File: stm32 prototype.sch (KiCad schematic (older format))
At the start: 117 parts, among them J1 USB_B_Mini, J3 Conn_01x02, Q1 Q_NMOS_GSD, Q2 Q_NMOS_GSD, Q3 Q_NMOS_GSD, Q4 Q_NMOS_GSD, Q5 Q_NMOS_GSD, Q6 Q_NMOS_GSD, Q7 Q_NMOS_GSD, Q8 Q_NMOS_GSD, Q9 Q_NMOS_GSD, U1 FT232RL, U2 W25Q128JV-DTR, U3 STM32F407VGTx, U4 LD1117S33TR, U5 ESP32, U6 IS25LP016D-JNLE-TR, Y1 Crystal_GND24, Y2 Crystal_GND23, Y3 Crystal_GND23

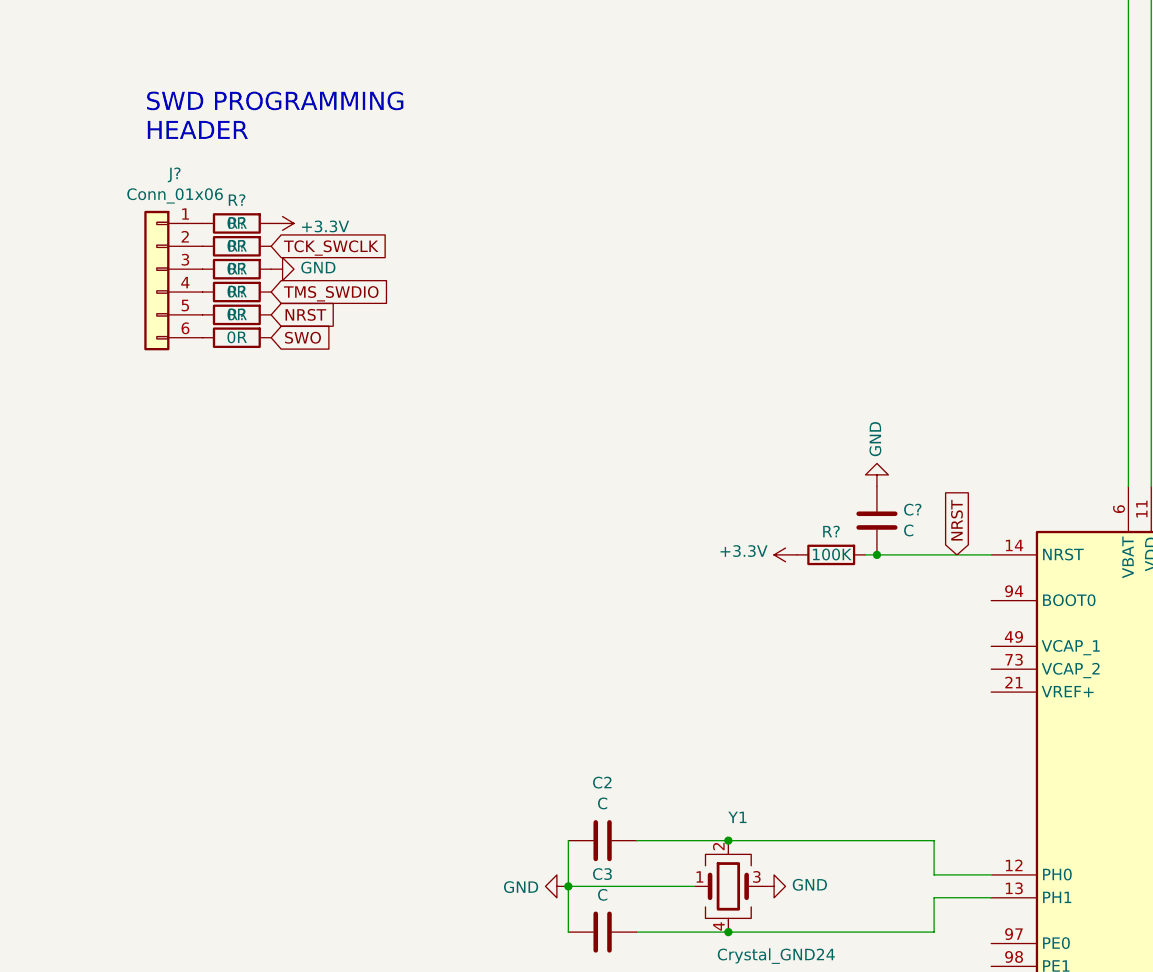
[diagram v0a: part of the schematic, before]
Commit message: worked on some layout
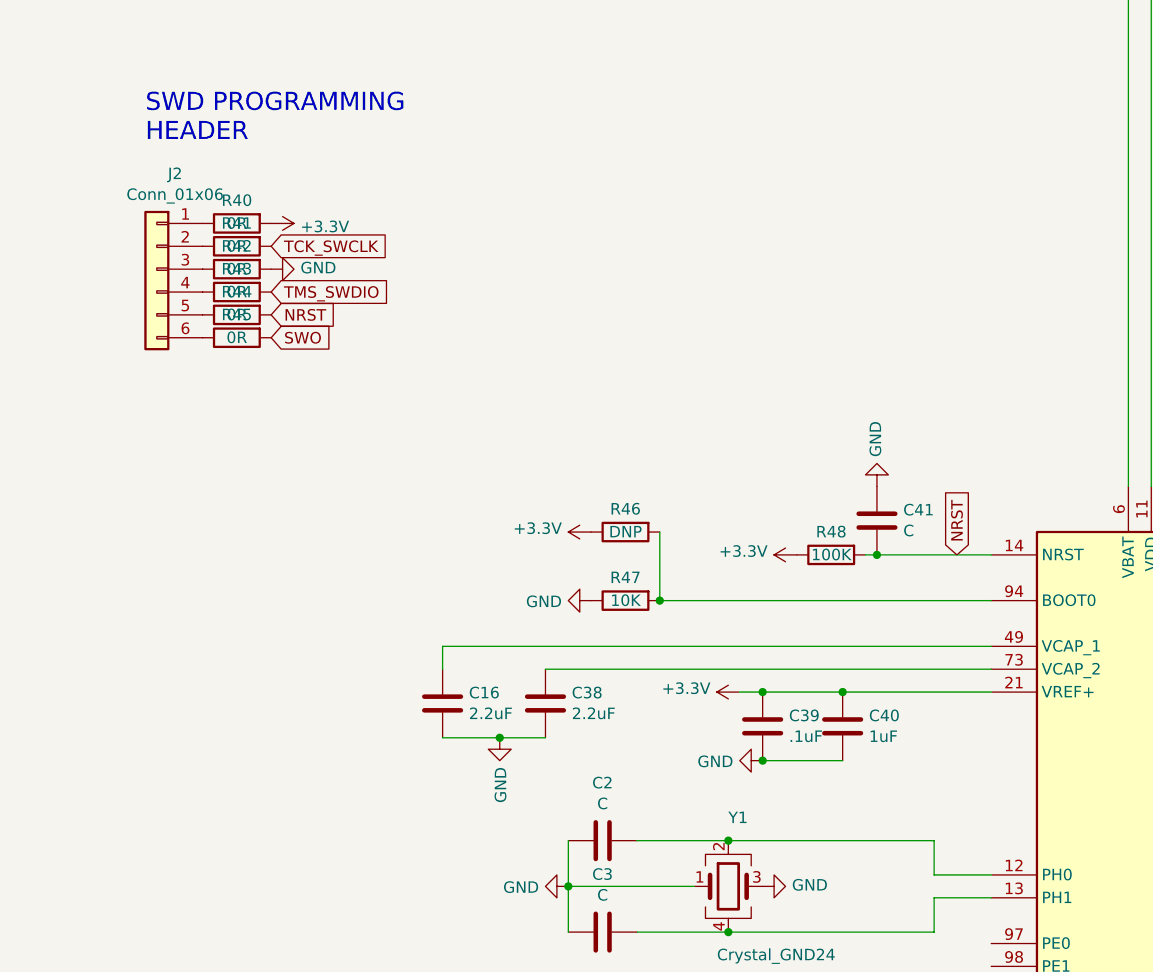
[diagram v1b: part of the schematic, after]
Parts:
- added C16, C38: 2.2uF, Capacitors_SMD:C_0603, symbol Device:C
- added C39: .1uF, Capacitors_SMD:C_0603, symbol Device:C
- added C40: 1uF, Capacitors_SMD:C_0603, symbol Device:C
- added R46: DNP, Resistors_SMD:R_0603, symbol Device:R
- added R47: 10K, Resistors_SMD:R_0603, symbol Device:R
- C1, C10, C11, C12, C13, C14, C15, C17, C18, C19, C2, C20, C21, C22, C23, C24, C25, C26, C27, C28, C29, C3, C31, C36, C37, C4, C5, C6, C7, C8, C9: footprint Capacitors_SMD:C_0603_HandSoldering -> Capacitors_SMD:C_0603
- C41: renamed from C?; footprint Capacitors_SMD:C_0603_HandSoldering -> Capacitors_SMD:C_0603
- D10, D11, D2, D3, D4, D5, D6, D7, D8, D9: footprint LEDs:LED_1206_HandSoldering -> LEDs:LED_1206
- Q1, Q2, Q3, Q4, Q5, Q6, Q7, Q8: footprint TO_SOT_Packages_SMD:SOT-323_SC-70_Handsoldering -> TO_SOT_Packages_SMD:SOT-323_SC-70
- R1, R10, R11, R12, R13, R14, R15, R16, R17, R18, R19, R2, R20, R21, R22, R23, R24, R25, R3, R34, R35, R36, R4, R5, R6, R7, R8, R9: footprint Resistors_SMD:R_0603_HandSoldering -> Resistors_SMD:R_0603
- R40, R41, R42, R43, R44, R45, R48: renamed from R?; footprint Resistors_SMD:R_0603_HandSoldering -> Resistors_SMD:R_0603
- gave numbers to parts that had none: 1
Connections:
- net +3V3: now also U3.21 (VREF+), C39.2, C40.2, R46.1
- net GND: now also C16.1, C38.1, C39.1, C40.1, R47.1
- net at U3.49 (VCAP_1): now also C16.2
- net at U3.73 (VCAP_2): now also C38.2
- net at U3.94 (BOOT0): now also R46.2, R47.2
